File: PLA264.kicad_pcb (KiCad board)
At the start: 2 copper layers, 18.3 x 37.1 mm, 10 parts, among them J1 PLA_Socket, U1 GAL16V8

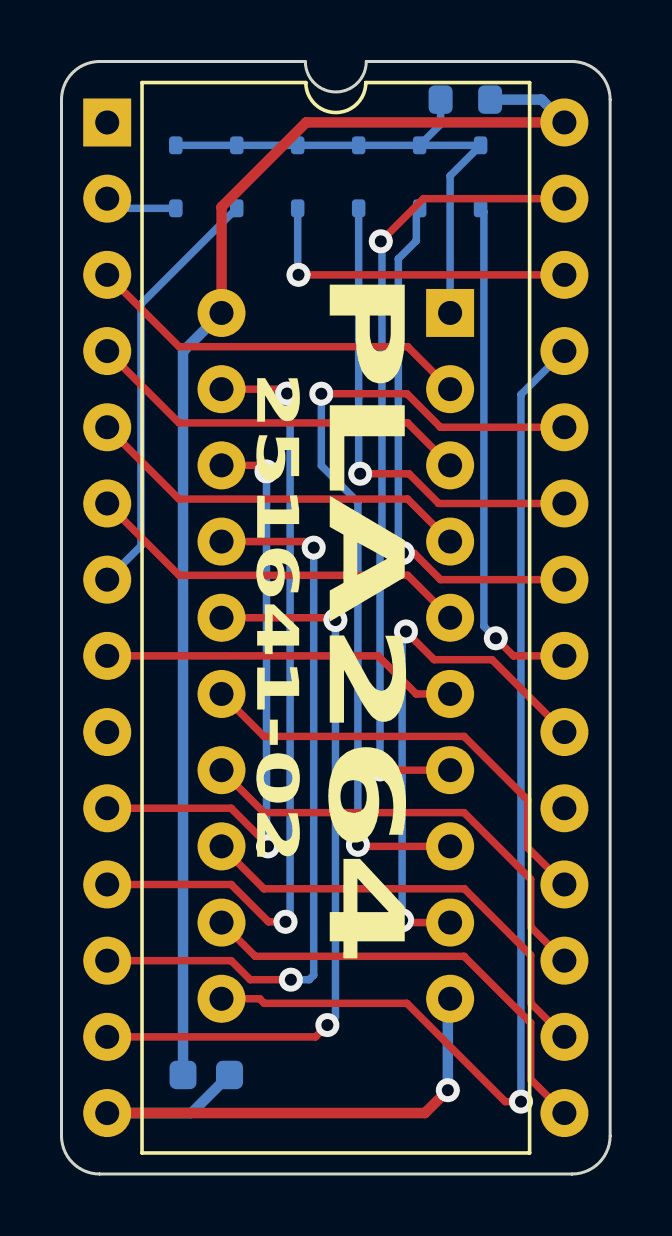
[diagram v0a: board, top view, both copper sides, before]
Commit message: Cleaning up.
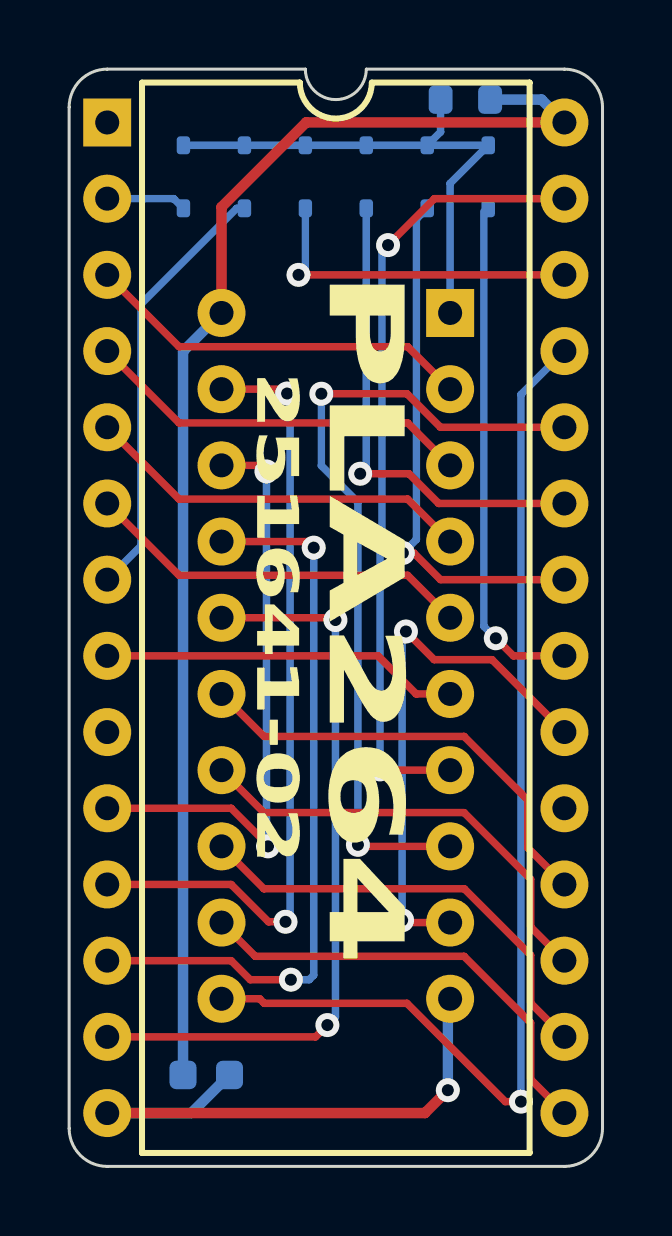
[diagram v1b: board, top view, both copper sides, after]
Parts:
- D1: renamed from D5; value D_Small -> 1N4148WS
- D2: renamed from D6; value D_Small -> 1N4148WS
- D3: renamed from D1; value D_Small -> 1N4148WS
- D4: renamed from D2; value D_Small -> 1N4148WS
- D5: renamed from D3; value D_Small -> 1N4148WS
- D6: renamed from D4; value D_Small -> 1N4148WS
- moved D1 0.25 mm to (99.1, 57.7)
- moved D2 0.25 mm to (101.1, 57.7)
- moved D4 0.25 mm to (105.2, 57.7)
- moved D5 0.25 mm to (107.2, 57.7)
- moved D6 0.25 mm to (109.2, 57.7)
- moved D3 0.25 mm to (103.1, 57.7)
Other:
- board size 18.3 x 37.1 mm -> 17.8 x 36.6 mm
- board text added: "github.com/hackup/PLA264"

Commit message: Preparing for Gerber export.
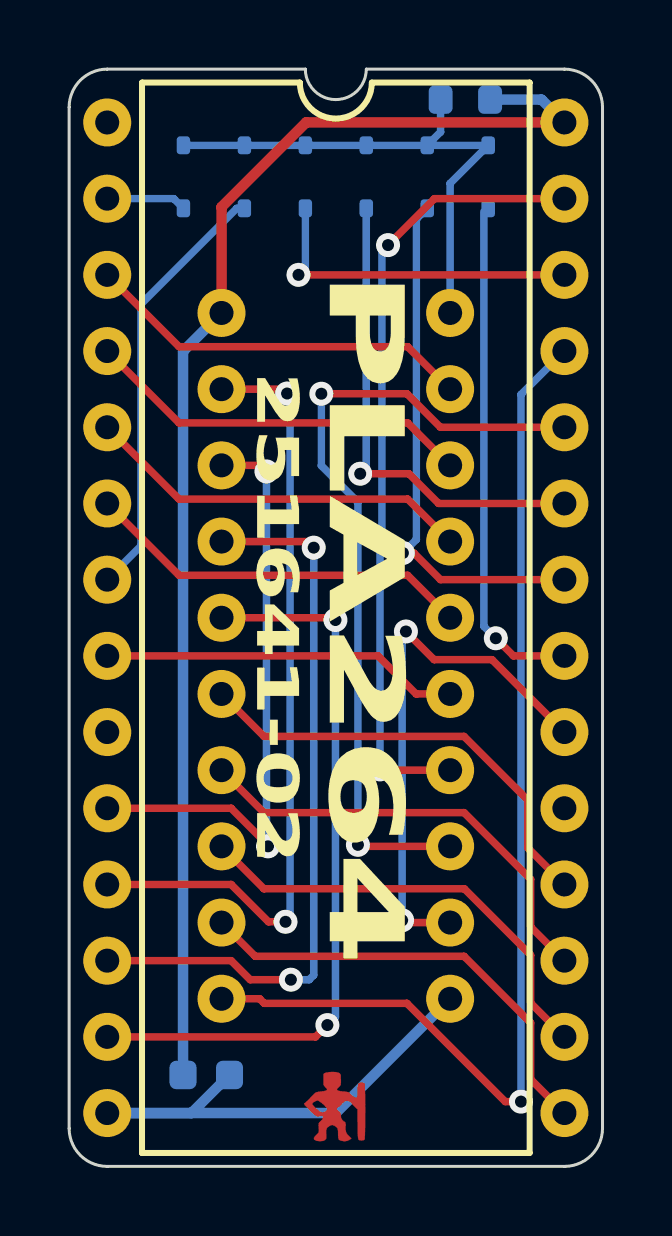
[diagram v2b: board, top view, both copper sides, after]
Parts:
- added G***: LOGO, Logo:bigby3-cu, F.Cu at (104.1, 88.6)
- R1: value R -> 5k6
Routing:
- net GND: track 19.4 -> 17.6 mm, vias 1 -> 0
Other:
- board text added: "PLA264 Rev.0"
